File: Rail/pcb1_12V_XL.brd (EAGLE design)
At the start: 96.3 x 101.8 mm, 116 parts, among them J1 638207222006, J10 638207222006, J11 638207222006, J12 638207222006, J2 638207222006, J4 61300421121, U1 ESP32-S3-DEVKITC-1-N8R2, U4 TLE9250VSJ, X2 B4P-VH

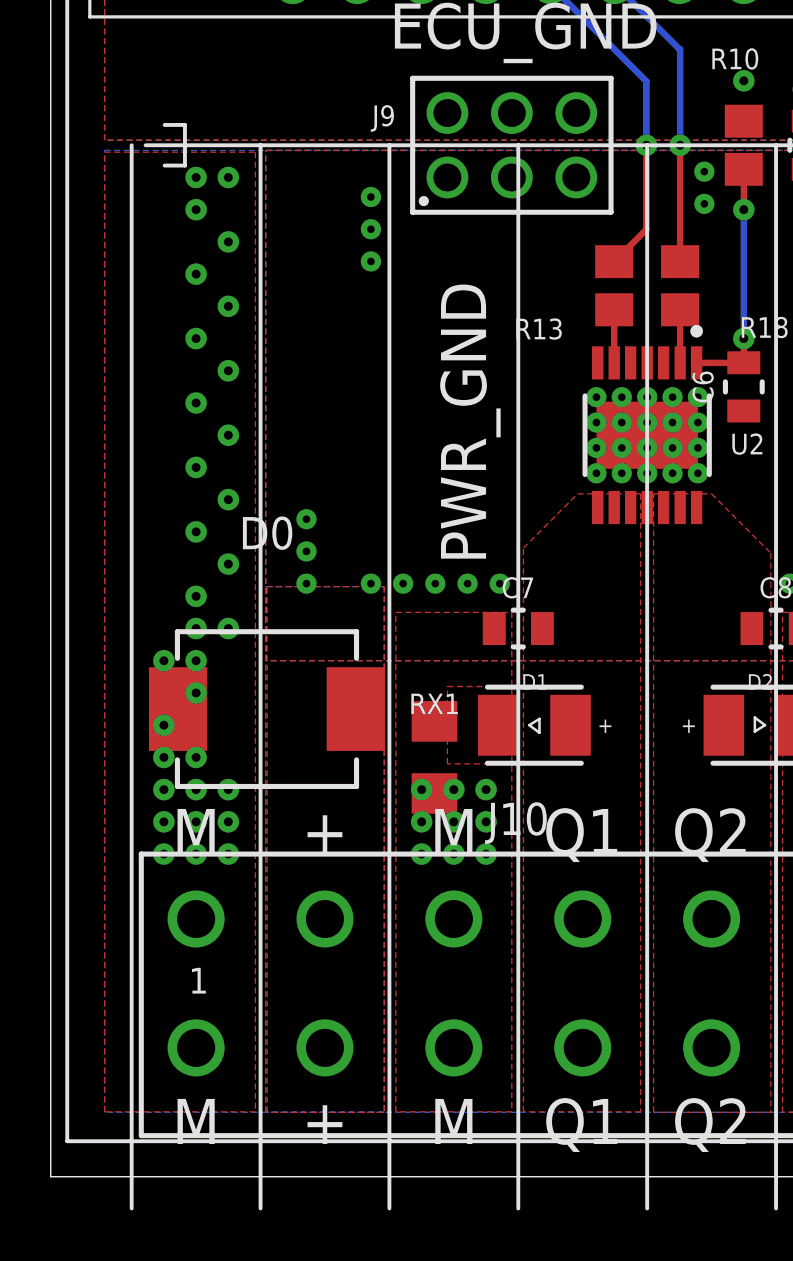
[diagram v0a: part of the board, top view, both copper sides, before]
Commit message: Order again
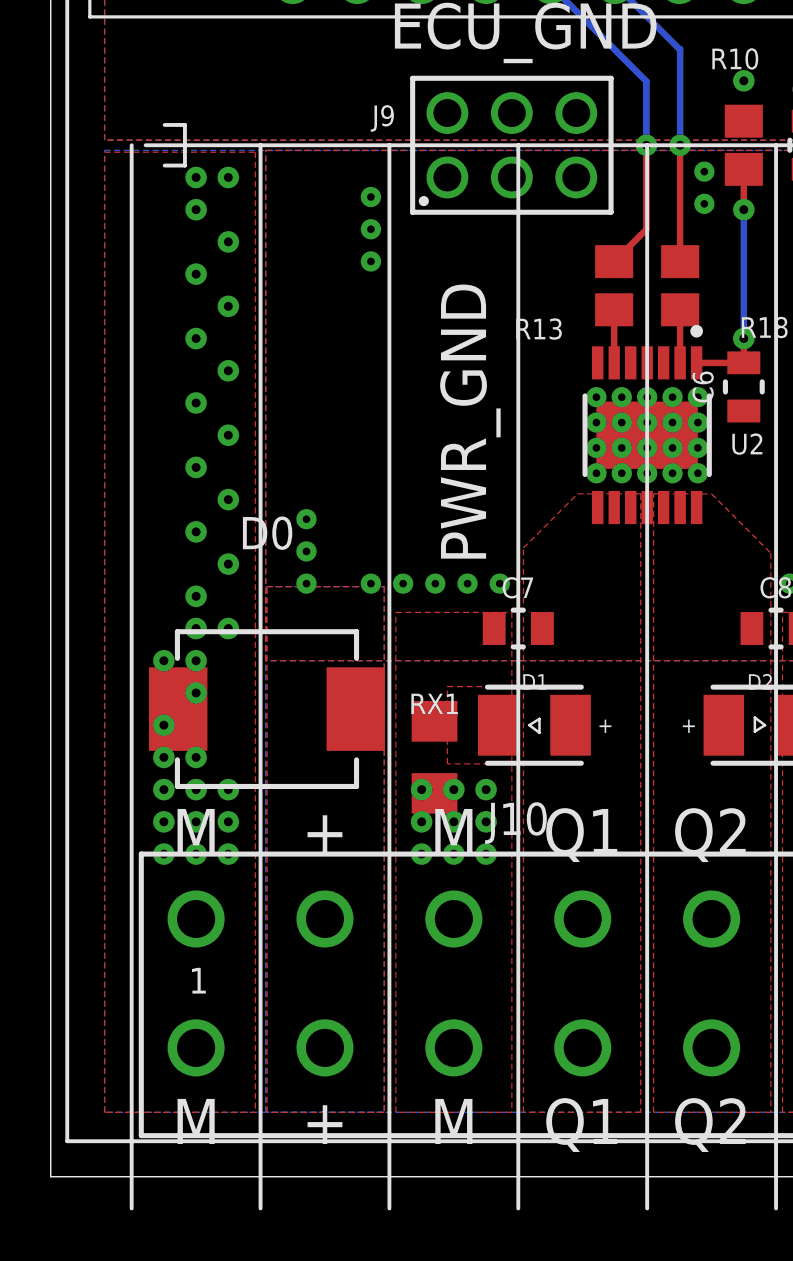
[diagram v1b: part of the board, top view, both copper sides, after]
